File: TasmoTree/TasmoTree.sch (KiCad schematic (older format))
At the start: 17 parts, among them J1 POWER_IN, J2 MOT_SW_CONN, J3 MOTOR_POWER, J4 LED_5MM_CONN, J5 LED_CONN_1, J6 LED_CONN_2, Q1 PSMN027-100PS, Q2 PSMN027-100PS, Q3 PSMN027-100PS, U1 ESP8266, U2 LD1117S33TR_SOT223, U3 LED-DRIVER, U4 LED-DRIVER, U5 LED-DRIVER

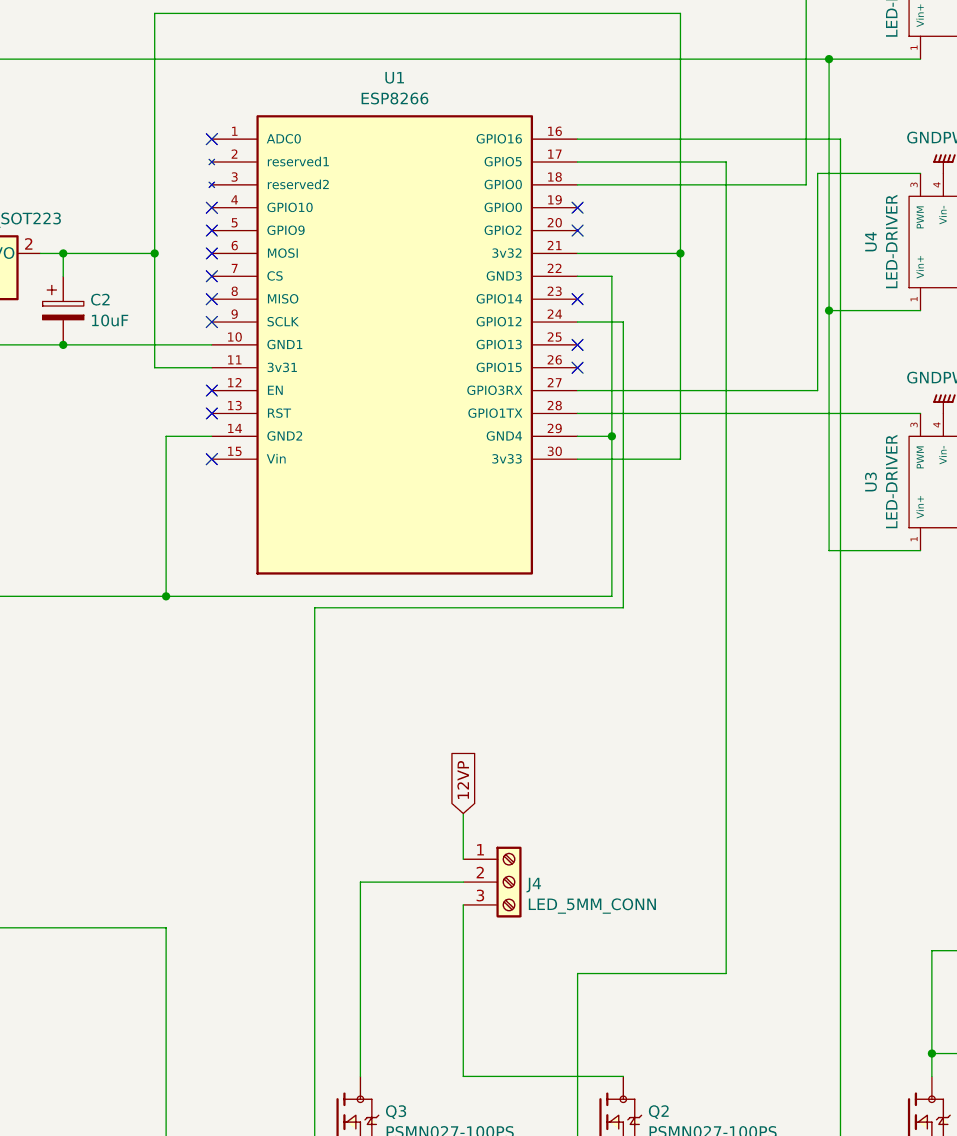
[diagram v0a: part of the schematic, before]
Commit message: added missing rotary encoder
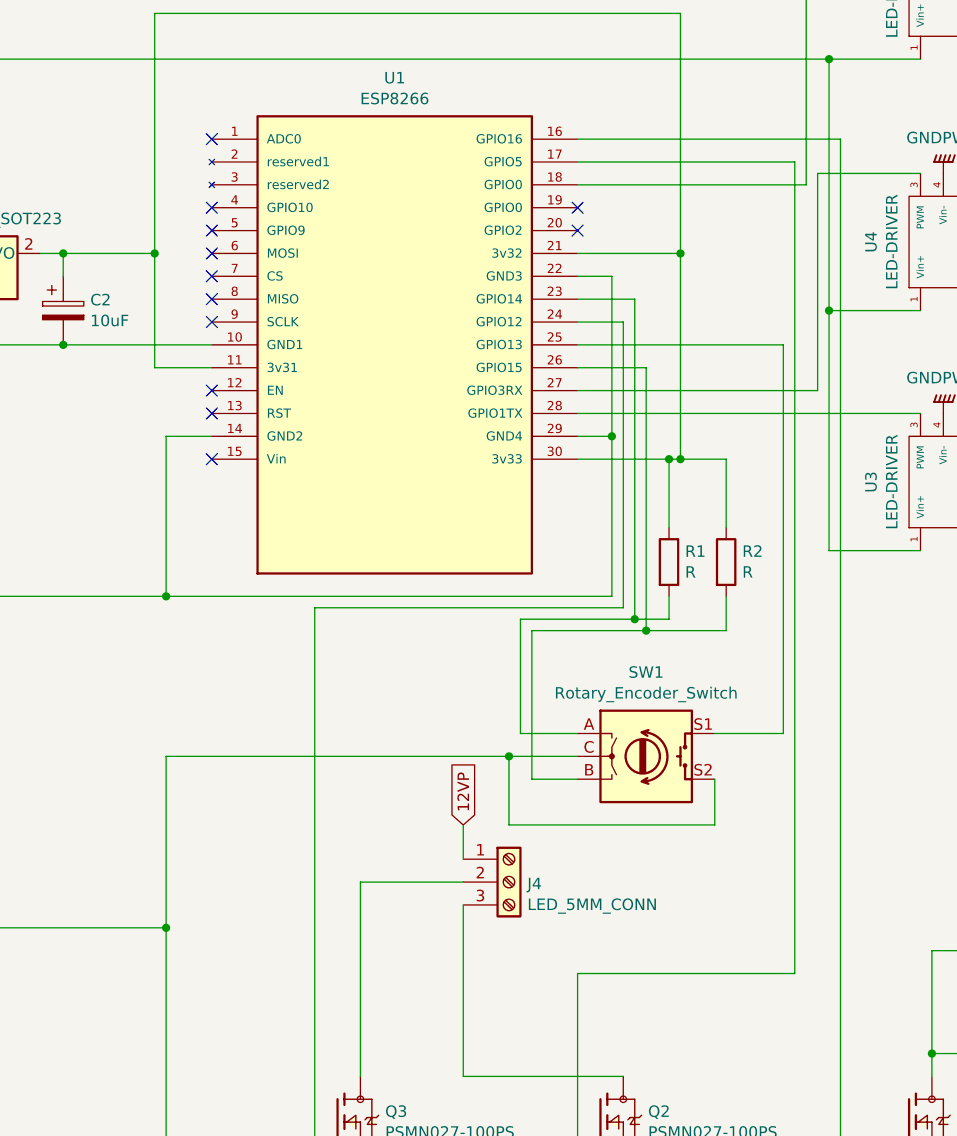
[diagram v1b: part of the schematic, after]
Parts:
- added R1, R2: R, symbol Device:R
- added SW1: Rotary_Encoder_Switch, symbol Device:Rotary_Encoder_Switch
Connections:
- net GNDPWR: now also SW1.C, SW1.S2
- net at C2.1, U1.11 (3v31), U1.21 (3v32)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: now also R1.1, R2.1
- net at U1.23 (GPIO14): now also R1.2, SW1.A
- net at U1.25 (GPIO13): now also SW1.S1
- net at U1.26 (GPIO15): now also R2.2, SW1.B
- no-connect marks 15 -> 12
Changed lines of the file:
@@
 Text Label 1150 1650 0    30   ~ 0
 32V
-$Comp
-L TasmoTree-rescue:ESP8266-DEVKIT U1
-U 1 1 5FC1B5D0
-P 3500 3200
-F 0 "U1" H 3500 4367 50  0000 C CNN
-F 1 "ESP8266" H 3500 4276 50  0000 C CNN
-F 2 "MODULE_ESP32-DEVKITC-32D" H 3500 3200 50  0001 L BNN
-F 3 "" H 3500 3200 50  0001 L BNN
-F 4 "4" H 3500 3200 50  0001 L BNN "PARTREV"
-F 5 "Espressif Systems" H 3500 3200 50  0001 L BNN "MANUFACTURER"
-	1    3500 3200
-	1    0    0    -1
-$EndComp
 Connection ~ 5850 6300
 Wire Wire Line
@@
 	3350 7300 4500 7300
 Wire Wire Line
-	4300 2400 4950 2400
-Wire Wire Line
-	4950 2400 4950 5950
-Wire Wire Line
-	4950 5950 4300 5950
+	5250 2400 5250 5950
 Wire Wire Line
 	4300 5950 4300 6700
@@
 	1    0    0    -1
 $EndComp
-Text GLabel 3800 5250 1    50   Input ~ 0
+Text GLabel 3800 5300 1    50   Input ~ 0
 12VP
-Wire Wire Line
-	3800 5450 3800 5250
 Wire Wire Line
 	3800 5550 3350 5550
@@
 	7050 1350 7050 2550
 Wire Wire Line
-	4300 3700 4750 3700
+	4300 3700 4700 3700
 Wire Wire Line
 	4750 3700 4750 2800
@@
 NoConn ~ 2700 3500
 NoConn ~ 2700 3700
-NoConn ~ 4300 3300
-NoConn ~ 4300 3200
-NoConn ~ 4300 3000
 NoConn ~ 4300 2700
 NoConn ~ 4300 2600
+$Comp
+L Device:Rotary_Encoder_Switch SW1
+U 1 1 5FD20C7F
+P 4600 5000
+F 0 "SW1" H 4600 5367 50  0000 C CNN
+F 1 "Rotary_Encoder_Switch" H 4600 5276 50  0000 C CNN
+F 2 "" H 4450 5160 50  0001 C CNN
+F 3 "~" H 4600 5260 50  0001 C CNN
+	1    4600 5000
+	1    0    0    -1
+$EndComp
+Wire Wire Line
+	4300 5950 5250 5950
+Wire Wire Line
+	4300 2400 5250 2400
+Wire Wire Line
+	5200 4900 5200 3200
+$Comp
+L TasmoTree-rescue:ESP8266-DEVKIT U1
+U 1 1 5FC1B5D0
+P 3500 3200
+F 0 "U1" H 3500 4367 50  0000 C CNN
+F 1 "ESP8266" H 3500 4276 50  0000 C CNN
+F 2 "MODULE_ESP32-DEVKITC-32D" H 3500 3200 50  0001 L BNN
+F 3 "" H 3500 3200 50  0001 L BNN
+F 4 "4" H 3500 3200 50  0001 L BNN "PARTREV"
+F 5 "Espressif Systems" H 3500 3200 50  0001 L BNN "MANUFACTURER"
+	1    3500 3200
+	1    0    0    -1
+$EndComp
+Wire Wire Line
+	4300 3000 4550 3000
+Wire Wire Line
+	4550 4400 4050 4400
+Wire Wire Line
+	4050 4400 4050 4900
+Wire Wire Line
+	4050 4900 4300 4900
+Wire Wire Line
+	4300 5100 4100 5100
+Wire Wire Line
+	4100 5100 4100 4450
+Wire Wire Line
+	4100 4450 4600 4450
+Wire Wire Line
+	4600 4450 4600 3300
+Wire Wire Line
+	4600 3300 4300 3300
+Wire Wire Line
+	4300 5000 4000 5000
+Wire Wire Line
+	2500 5000 2500 5750
+Connection ~ 2500 5750
+Wire Wire Line
+	4000 5000 4000 5300
+Wire Wire Line
+	4000 5300 4900 5300
+Wire Wire Line
+	4900 5300 4900 5100
+Connection ~ 4000 5000
+Wire Wire Line
+	4000 5000 2500 5000
+Wire Wire Line
+	3800 5450 3800 5300
+$Comp
+L Device:R R1
+U 1 1 5FD60931
+P 4700 4150
+F 0 "R1" H 4770 4196 50  0000 L CNN
+F 1 "R" H 4770 4105 50  0000 L CNN
+F 2 "" V 4630 4150 50  0001 C CNN
+F 3 "~" H 4700 4150 50  0001 C CNN
+	1    4700 4150
+	1    0    0    -1
+$EndComp
+$Comp
+L Device:R R2
+U 1 1 5FD612A1
+P 4950 4150
+F 0 "R2" H 5020 4196 50  0000 L CNN
+F 1 "R" H 5020 4105 50  0000 L CNN
+F 2 "" V 4880 4150 50  0001 C CNN
+F 3 "~" H 4950 4150 50  0001 C CNN
+	1    4950 4150
+	1    0    0    -1
+$EndComp
+Wire Wire Line
+	4700 4000 4700 3700
+Connection ~ 4700 3700
+Wire Wire Line
+	4700 3700 4750 3700
+Wire Wire Line
+	4750 3700 4950 3700
+Wire Wire Line
+	4950 3700 4950 4000
+Connection ~ 4750 3700
+Wire Wire Line
+	4950 4300 4950 4450
+Wire Wire Line
+	4950 4450 4600 4450
+Connection ~ 4600 4450
+Wire Wire Line
+	4550 4400 4700 4400
+Wire Wire Line
+	4700 4400 4700 4300
+Connection ~ 4550 4400
+Wire Wire Line
+	4550 3000 4550 4400
+Wire Wire Line
+	4900 4900 5200 4900
+Wire Wire Line
+	4300 3200 5200 3200
 $EndSCHEMATC

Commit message: rough design of pcb layout added
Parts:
- C1: footprint (none) -> Capacitors_THT:C_Disc_D3.0mm_W1.6mm_P2.50mm
- C2: footprint (none) -> Capacitors_THT:CP_Radial_D4.0mm_P1.50mm
- J1: footprint (none) -> Connectors_Terminal_Blocks:TerminalBlock_Altech_AK300-4_P5.00mm
- J2, J4, J5, J6: footprint (none) -> Connectors_Terminal_Blocks:TerminalBlock_Altech_AK300-3_P5.00mm
- J3: footprint (none) -> Connectors_Terminal_Blocks:TerminalBlock_Altech_AK300-2_P5.00mm
- Q1, Q2, Q3: footprint TO255P1040X460X2890-3 -> TasmoTree:TO255P1040X460X2890-3
- R1, R2: footprint (none) -> Resistors_Universal:Resistor_SMD+THTuniversal_0805to1206_RM10_HandSoldering
- S1: footprint RELAY_7-1393243-9 -> TasmoTree:RELAY_7-1393243-9
- SW1: footprint (none) -> TasmoTree:XDCR_PEC11R-4215F-S0024; symbol Device:Rotary_Encoder_Switch -> TasmoTree:PEC11R-4215F-S0024
- U1: footprint MODULE_ESP32-DEVKITC-32D -> TasmoTree:MODULE_ESP32-DEVKITC-32D
- U2: footprint Package_TO_SOT_SMD:SOT-223-3_TabPin2 -> TO_SOT_Packages_THT:TO-220-3_Vertical
- U3, U4, U5: footprint (none) -> TasmoTree:LDD-L-MEANWELL
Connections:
- net GNDPWR: now also SW1.1, SW1.COM, SW1.S1 (SHIELD); no longer SW1.C
- net at R1.2, SW1.A: now also U1.26 (GPIO15); no longer U1.23 (GPIO14)
- net at U1.25 (GPIO13): now also R2.2, SW1.2; no longer SW1.S1
- new net: SW1.B, U1.23 (GPIO14)
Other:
- moved on the sheet: R1, R2
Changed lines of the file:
@@
 F 0 "U2" H 1650 3042 50  0000 C CNN
 F 1 "LD1117S33TR_SOT223" H 1650 2951 50  0000 C CNN
-F 2 "Package_TO_SOT_SMD:SOT-223-3_TabPin2" H 1650 3000 50  0001 C CNN
+F 2 "TO_SOT_Packages_THT:TO-220-3_Vertical" H 1650 3000 50  0001 C CNN
 F 3 "http://www.st.com/st-web-ui/static/active/en/resource/technical/document/datasheet/CD00000544.pdf" H 1750 2550 50  0001 C CNN
 	1    1650 2800
@@
 F 0 "C1" H 1265 3096 50  0000 L CNN
 F 1 "100nF" H 1265 3005 50  0000 L CNN
-F 2 "" H 1188 2900 50  0001 C CNN
+F 2 "Capacitors_THT:C_Disc_D3.0mm_W1.6mm_P2.50mm" H 1188 2900 50  0001 C CNN
 F 3 "~" H 1150 3050 50  0001 C CNN
 	1    1150 3050
@@
 F 0 "C2" H 2168 3096 50  0000 L CNN
 F 1 "10uF" H 2168 3005 50  0000 L CNN
-F 2 "" H 2088 2900 50  0001 C CNN
+F 2 "Capacitors_THT:CP_Radial_D4.0mm_P1.50mm" H 2088 2900 50  0001 C CNN
 F 3 "~" H 2050 3050 50  0001 C CNN
 	1    2050 3050
@@
 F 0 "S1" H 7150 6217 50  0000 C CNN
 F 1 "EC2-12NU" H 7150 6126 50  0000 C CNN
-F 2 "RELAY_7-1393243-9" H 7150 5450 50  0001 L BNN
+F 2 "TasmoTree:RELAY_7-1393243-9" H 7150 5450 50  0001 L BNN
 F 3 "" H 7150 5450 50  0001 L BNN
 F 4 "7-1393243-9" H 7150 5450 50  0001 L BNN "Comment"
@@
 F 0 "Q1" H 5958 6646 50  0000 L CNN
 F 1 "PSMN027-100PS" H 5958 6555 50  0000 L CNN
-F 2 "TO255P1040X460X2890-3" H 5750 6600 50  0001 L BNN
+F 2 "TasmoTree:TO255P1040X460X2890-3" H 5750 6600 50  0001 L BNN
 F 3 "" H 5750 6600 50  0001 L BNN
 F 4 "IPC-7251" H 5750 6600 50  0001 L BNN "STANDARD"
@@
 F 0 "U5" H 5650 1715 50  0000 C CNN
 F 1 "LED-DRIVER" H 5650 1624 50  0000 C CNN
-F 2 "" H 5600 1700 50  0001 C CNN
+F 2 "TasmoTree:LDD-L-MEANWELL" H 5600 1700 50  0001 C CNN
 F 3 "" H 5600 1700 50  0001 C CNN
 	1    5650 1650
@@
 F 0 "Q2" H 4608 6646 50  0000 L CNN
 F 1 "PSMN027-100PS" H 4608 6555 50  0000 L CNN
-F 2 "TO255P1040X460X2890-3" H 4400 6600 50  0001 L BNN
+F 2 "TasmoTree:TO255P1040X460X2890-3" H 4400 6600 50  0001 L BNN
 F 3 "" H 4400 6600 50  0001 L BNN
 F 4 "IPC-7251" H 4400 6600 50  0001 L BNN "STANDARD"
@@
 F 0 "J1" V 1014 1462 50  0000 R CNN
 F 1 "POWER_IN" V 923 1462 50  0000 R CNN
-F 2 "" H 1050 1750 50  0001 C CNN
+F 2 "Connectors_Terminal_Blocks:TerminalBlock_Altech_AK300-4_P5.00mm" H 1050 1750 50  0001 C CNN
 F 3 "~" H 1050 1750 50  0001 C CNN
 	1    1050 1750
@@
 F 0 "J2" H 8630 5042 50  0000 L CNN
 F 1 "MOT_SW_CONN" H 8630 4951 50  0000 L CNN
-F 2 "" H 8550 5050 50  0001 C CNN
+F 2 "Connectors_Terminal_Blocks:TerminalBlock_Altech_AK300-3_P5.00mm" H 8550 5050 50  0001 C CNN
 F 3 "~" H 8550 5050 50  0001 C CNN
 	1    8550 5050
@@
 F 0 "J3" H 8630 5442 50  0000 L CNN
 F 1 "MOTOR_POWER" H 8630 5351 50  0000 L CNN
-F 2 "" H 8550 5450 50  0001 C CNN
+F 2 "Connectors_Terminal_Blocks:TerminalBlock_Altech_AK300-2_P5.00mm" H 8550 5450 50  0001 C CNN
 F 3 "~" H 8550 5450 50  0001 C CNN
 	1    8550 5450
@@
 F 0 "U4" H 5650 2815 50  0000 C CNN
 F 1 "LED-DRIVER" H 5650 2724 50  0000 C CNN
-F 2 "" H 5600 2800 50  0001 C CNN
+F 2 "TasmoTree:LDD-L-MEANWELL" H 5600 2800 50  0001 C CNN
 F 3 "" H 5600 2800 50  0001 C CNN
 	1    5650 2750
@@
 F 0 "U3" H 5650 3865 50  0000 C CNN
 F 1 "LED-DRIVER" H 5650 3774 50  0000 C CNN
-F 2 "" H 5600 3850 50  0001 C CNN
+F 2 "TasmoTree:LDD-L-MEANWELL" H 5600 3850 50  0001 C CNN
 F 3 "" H 5600 3850 50  0001 C CNN
 	1    5650 3800
@@
 F 0 "Q3" H 3458 6646 50  0000 L CNN
 F 1 "PSMN027-100PS" H 3458 6555 50  0000 L CNN
-F 2 "TO255P1040X460X2890-3" H 3250 6600 50  0001 L BNN
+F 2 "TasmoTree:TO255P1040X460X2890-3" H 3250 6600 50  0001 L BNN
 F 3 "" H 3250 6600 50  0001 L BNN
 F 4 "IPC-7251" H 3250 6600 50  0001 L BNN "STANDARD"
@@
 F 0 "J4" H 4080 5542 50  0000 L CNN
 F 1 "LED_5MM_CONN" H 4080 5451 50  0000 L CNN
-F 2 "" H 4000 5550 50  0001 C CNN
+F 2 "Connectors_Terminal_Blocks:TerminalBlock_Altech_AK300-3_P5.00mm" H 4000 5550 50  0001 C CNN
 F 3 "~" H 4000 5550 50  0001 C CNN
 	1    4000 5550
@@
 F 0 "J6" H 7330 3042 50  0000 L CNN
 F 1 "LED_CONN_2" H 7330 2951 50  0000 L CNN
-F 2 "" H 7250 3050 50  0001 C CNN
+F 2 "Connectors_Terminal_Blocks:TerminalBlock_Altech_AK300-3_P5.00mm" H 7250 3050 50  0001 C CNN
 F 3 "~" H 7250 3050 50  0001 C CNN
 	1    7250 3050
@@
 F 0 "J5" H 7330 2642 50  0000 L CNN
 F 1 "LED_CONN_1" H 7330 2551 50  0000 L CNN
-F 2 "" H 7250 2650 50  0001 C CNN
+F 2 "Connectors_Terminal_Blocks:TerminalBlock_Altech_AK300-3_P5.00mm" H 7250 2650 50  0001 C CNN
 F 3 "~" H 7250 2650 50  0001 C CNN
 	1    7250 2650
@@
 	7050 1350 7050 2550
 Wire Wire Line
-	4300 3700 4700 3700
+	4300 3700 4600 3700
 Wire Wire Line
 	4750 3700 4750 2800
@@
 NoConn ~ 4300 2700
 NoConn ~ 4300 2600
-$Comp
-L Device:Rotary_Encoder_Switch SW1
+Wire Wire Line
+	4300 5950 5250 5950
+Wire Wire Line
+	4300 2400 5250 2400
+Wire Wire Line
+	2500 5000 2500 5750
+Connection ~ 2500 5750
+Wire Wire Line
+	3800 5450 3800 5300
+$Comp
+L Device:R R1
+U 1 1 5FD60931
+P 4600 4150
+F 0 "R1" H 4670 4196 50  0000 L CNN
+F 1 "R" H 4670 4105 50  0000 L CNN
+F 2 "Resistors_Universal:Resistor_SMD+THTuniversal_0805to1206_RM10_HandSoldering" V 4530 4150 50  0001 C CNN
+F 3 "~" H 4600 4150 50  0001 C CNN
+	1    4600 4150
+	1    0    0    -1
+$EndComp
+$Comp
+L Device:R R2
+U 1 1 5FD612A1
+P 4900 4000
+F 0 "R2" H 4970 4046 50  0000 L CNN
+F 1 "R" H 4970 3955 50  0000 L CNN
+F 2 "Resistors_Universal:Resistor_SMD+THTuniversal_0805to1206_RM10_HandSoldering" V 4830 4000 50  0001 C CNN
+F 3 "~" H 4900 4000 50  0001 C CNN
+	1    4900 4000
+	0    -1   -1   0
+$EndComp
+Wire Wire Line
+	4600 4000 4600 3700
+Wire Wire Line
+	4750 3700 4750 4000
+Connection ~ 4750 3700
+Wire Wire Line
+	4300 3200 5200 3200
+Wire Wire Line
+	4000 5100 4000 5000
+Connection ~ 4000 5000
+Wire Wire Line
+	4000 4800 4000 5000
+Wire Wire Line
+	4000 5000 2500 5000
+$Comp
+L TasmoTree:PEC11R-4215F-S0024 SW1
 U 1 1 5FD20C7F
-P 4600 5000
-F 0 "SW1" H 4600 5367 50  0000 C CNN
-F 1 "Rotary_Encoder_Switch" H 4600 5276 50  0000 C CNN
-F 2 "" H 4450 5160 50  0001 C CNN
-F 3 "~" H 4600 5260 50  0001 C CNN
-	1    4600 5000
-	1    0    0    -1
-$EndComp
-Wire Wire Line
-	4300 5950 5250 5950
-Wire Wire Line
-	4300 2400 5250 2400
-Wire Wire Line
-	5200 4900 5200 3200
+P 4400 4900
+F 0 "SW1" H 4400 5267 50  0000 C CNN
+F 1 "Rotary_Encoder_Switch" H 4400 5176 50  0000 C CNN
+F 2 "TasmoTree:XDCR_PEC11R-4215F-S0024" H 4250 5060 50  0001 C CNN
+F 3 "~" H 4400 5160 50  0001 C CNN
+	1    4400 4900
+	1    0    0    -1
+$EndComp
+Wire Wire Line
+	4800 4800 5200 4800
+Wire Wire Line
+	5200 4800 5200 4000
+Wire Wire Line
+	4800 5100 5150 5100
+Connection ~ 4600 3700
+Wire Wire Line
+	4600 3700 4750 3700
+Wire Wire Line
+	5150 3000 5150 5100
+Wire Wire Line
+	4300 3000 5150 3000
+Wire Wire Line
+	5050 4000 5200 4000
+Connection ~ 5200 4000
+Wire Wire Line
+	5200 4000 5200 3200
 $Comp
 L TasmoTree-rescue:ESP8266-DEVKIT U1
@@
 F 0 "U1" H 3500 4367 50  0000 C CNN
 F 1 "ESP8266" H 3500 4276 50  0000 C CNN
-F 2 "MODULE_ESP32-DEVKITC-32D" H 3500 3200 50  0001 L BNN
+F 2 "TasmoTree:MODULE_ESP32-DEVKITC-32D" H 3500 3200 50  0001 L BNN
 F 3 "" H 3500 3200 50  0001 L BNN
 F 4 "4" H 3500 3200 50  0001 L BNN "PARTREV"
@@
 $EndComp
 Wire Wire Line
-	4300 3000 4550 3000
-Wire Wire Line
-	4550 4400 4050 4400
-Wire Wire Line
-	4050 4400 4050 4900
-Wire Wire Line
-	4050 4900 4300 4900
-Wire Wire Line
-	4300 5100 4100 5100
-Wire Wire Line
-	4100 5100 4100 4450
-Wire Wire Line
-	4100 4450 4600 4450
-Wire Wire Line
-	4600 4450 4600 3300
-Wire Wire Line
-	4600 3300 4300 3300
-Wire Wire Line
-	4300 5000 4000 5000
-Wire Wire Line
-	2500 5000 2500 5750
-Connection ~ 2500 5750
-Wire Wire Line
-	4000 5000 4000 5300
-Wire Wire Line
-	4000 5300 4900 5300
-Wire Wire Line
-	4900 5300 4900 5100
-Connection ~ 4000 5000
-Wire Wire Line
-	4000 5000 2500 5000
-Wire Wire Line
-	3800 5450 3800 5300
-$Comp
-L Device:R R1
-U 1 1 5FD60931
-P 4700 4150
-F 0 "R1" H 4770 4196 50  0000 L CNN
-F 1 "R" H 4770 4105 50  0000 L CNN
-F 2 "" V 4630 4150 50  0001 C CNN
-F 3 "~" H 4700 4150 50  0001 C CNN
-	1    4700 4150
-	1    0    0    -1
-$EndComp
-$Comp
-L Device:R R2
-U 1 1 5FD612A1
-P 4950 4150
-F 0 "R2" H 5020 4196 50  0000 L CNN
-F 1 "R" H 5020 4105 50  0000 L CNN
-F 2 "" V 4880 4150 50  0001 C CNN
-F 3 "~" H 4950 4150 50  0001 C CNN
-	1    4950 4150
-	1    0    0    -1
-$EndComp
-Wire Wire Line
-	4700 4000 4700 3700
-Connection ~ 4700 3700
-Wire Wire Line
-	4700 3700 4750 3700
-Wire Wire Line
-	4750 3700 4950 3700
-Wire Wire Line
-	4950 3700 4950 4000
-Connection ~ 4750 3700
-Wire Wire Line
-	4950 4300 4950 4450
-Wire Wire Line
-	4950 4450 4600 4450
-Connection ~ 4600 4450
-Wire Wire Line
-	4550 4400 4700 4400
-Wire Wire Line
-	4700 4400 4700 4300
-Connection ~ 4550 4400
-Wire Wire Line
-	4550 3000 4550 4400
-Wire Wire Line
-	4900 4900 5200 4900
-Wire Wire Line
-	4300 3200 5200 3200
+	4300 3300 5100 3300
+Wire Wire Line
+	5100 3300 5100 4300
+Wire Wire Line
+	5100 5000 4800 5000
+Wire Wire Line
+	4600 4300 5100 4300
+Connection ~ 5100 4300
+Wire Wire Line
+	5100 4300 5100 5000
 $EndSCHEMATC

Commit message: bumped to KiCAD 5+, added workflow for test
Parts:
- U3, U4, U5: symbol TasmoTree:LED-DRIVER -> TasmoTree-rescue:LED-DRIVER-TasmoTree
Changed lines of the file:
@@
 	5850 7300 5850 6800
 $Comp
-L TasmoTree:LED-DRIVER U5
+L TasmoTree-rescue:LED-DRIVER-TasmoTree U5
 U 1 1 5FC8124B
 P 5650 1650
@@
 	8000 5550 8000 5950
 $Comp
-L TasmoTree:LED-DRIVER U4
+L TasmoTree-rescue:LED-DRIVER-TasmoTree U4
 U 1 1 5FC7CA67
 P 5650 2750
@@
 $EndComp
 $Comp
-L TasmoTree:LED-DRIVER U3
+L TasmoTree-rescue:LED-DRIVER-TasmoTree U3
 U 1 1 5FC82B1A
 P 5650 3800
